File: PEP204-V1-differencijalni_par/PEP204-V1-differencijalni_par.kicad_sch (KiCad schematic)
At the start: 18 parts, among them J1 Screw_Terminal_01x02, J2 Conn_01x02_Pin, J3 Conn_01x02_Pin, J4 Conn_01x02_Pin, J5 Conn_01x02_Pin, Q1 MMBT2222A, Q2 MMBT2222A, Q3 MMBT2222A, U1 CJ432

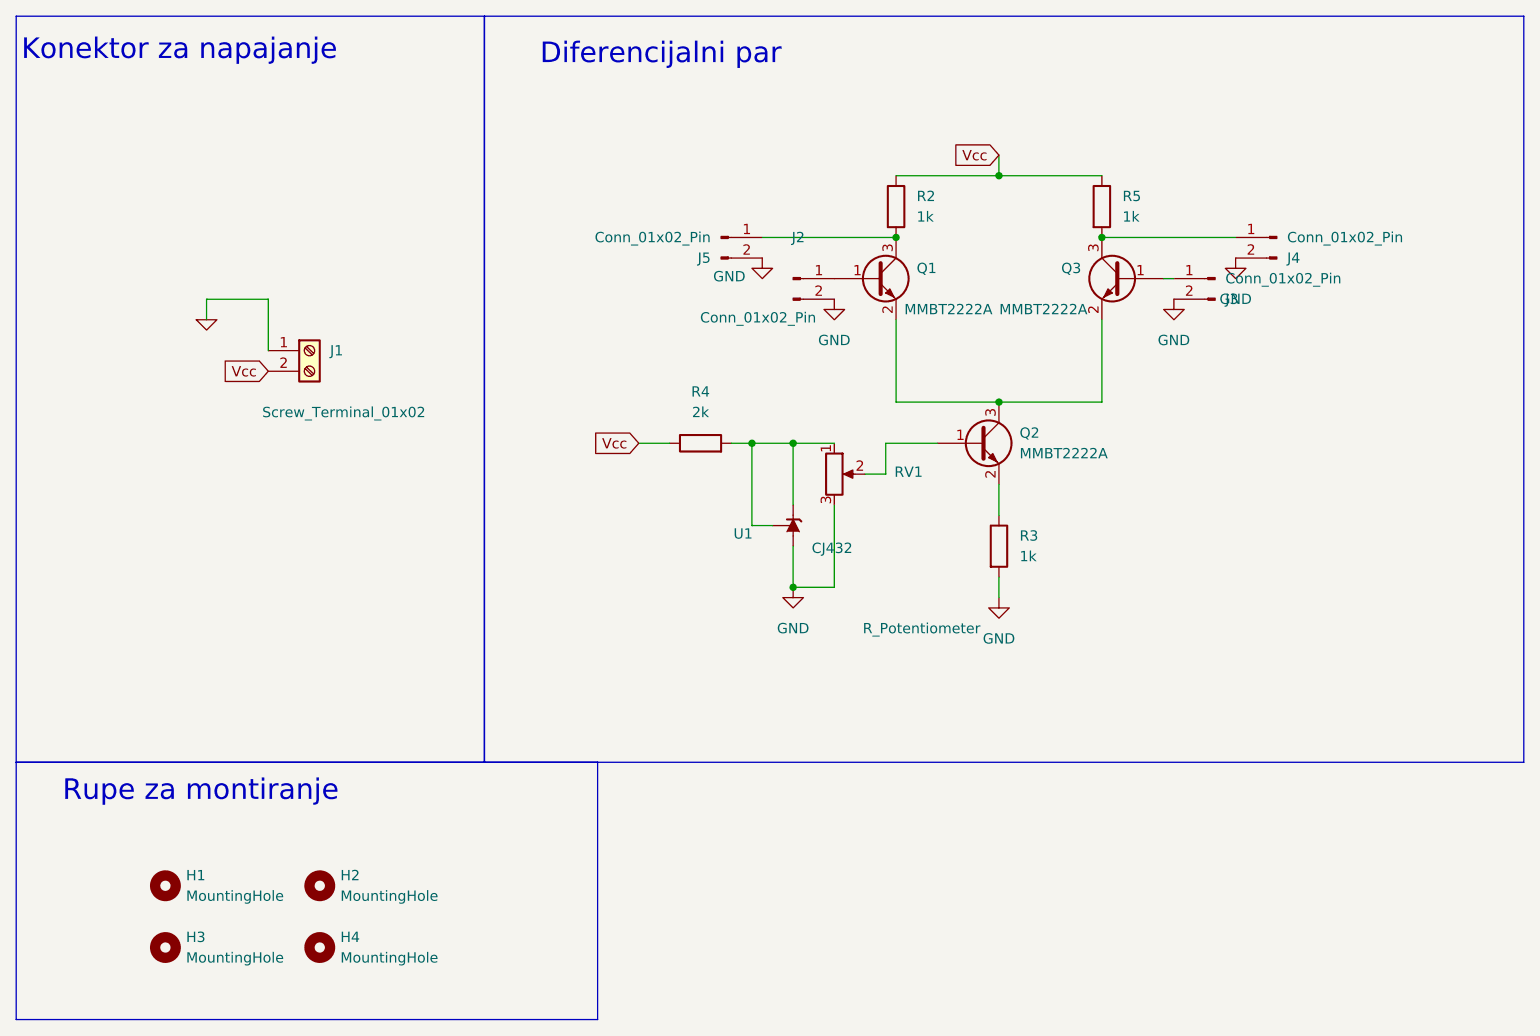
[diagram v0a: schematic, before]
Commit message: PEP201 i PEP204 :)
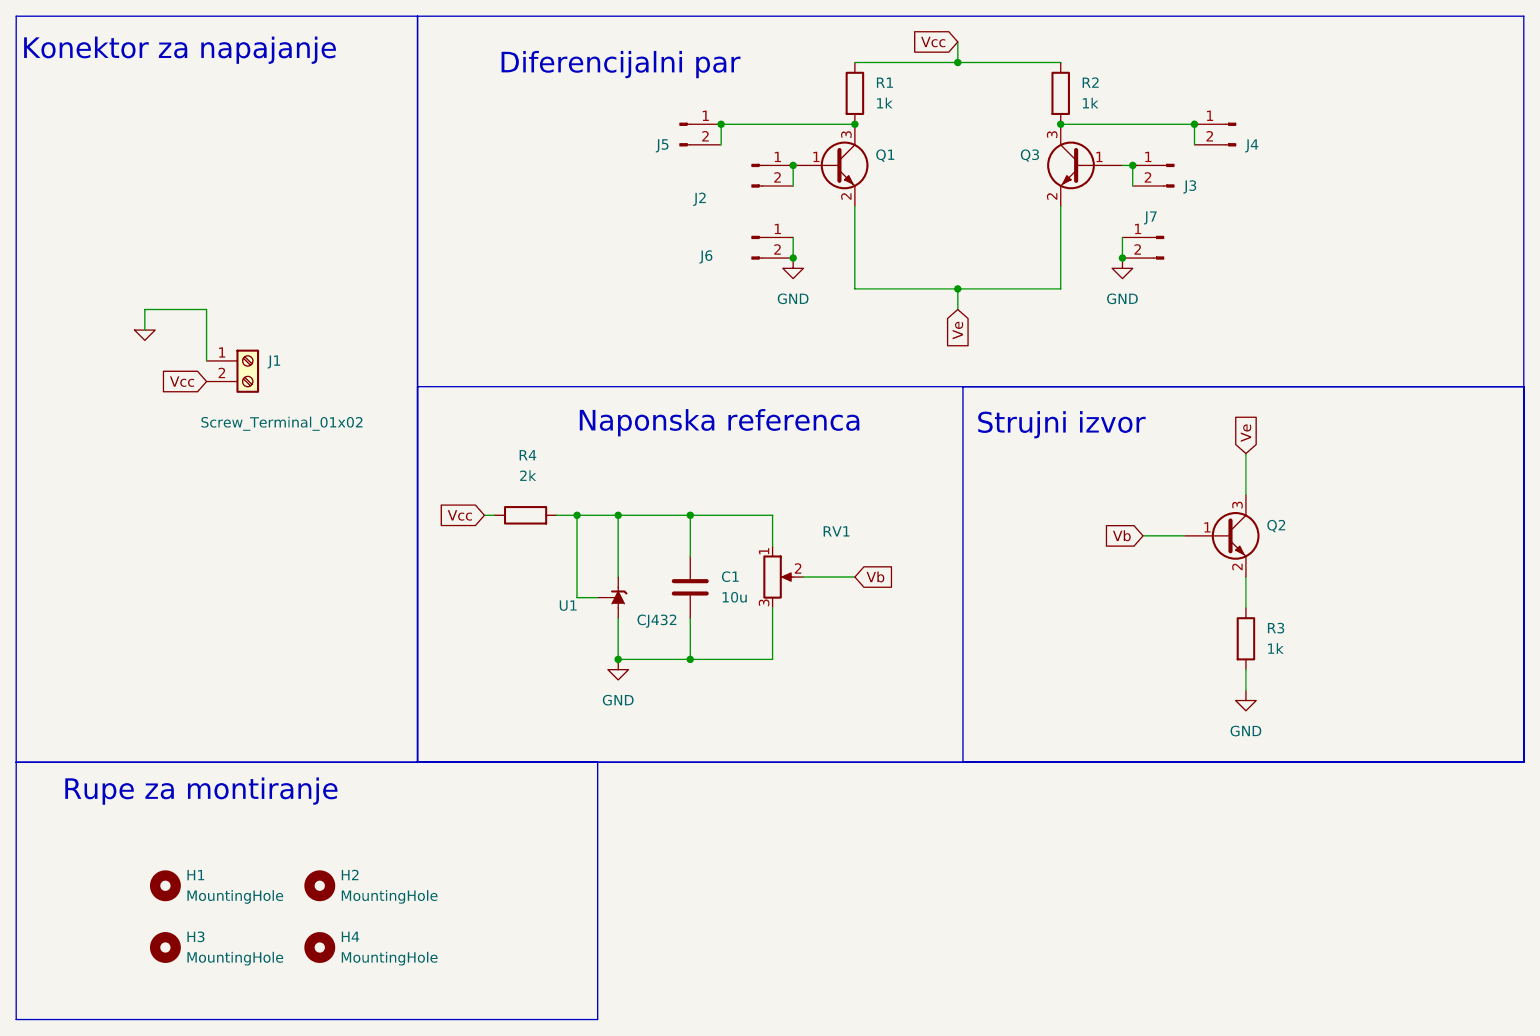
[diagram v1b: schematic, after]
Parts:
- added C1: 10u, PEP_library:C_1206_3216Metric, symbol Device:C
- added J6, J7: Conn_01x02_Pin, PEP_library:PinHeader_1x02_P2.54mm_Vertical, symbol Connector:Conn_01x02_Pin
- Q1, Q2, Q3: LCSC (none) -> C8512
- R1: renamed from R2; LCSC (none) -> C4410
- R2: renamed from R5; LCSC (none) -> C4410
- R3: LCSC (none) -> C4410
- R4: LCSC (none) -> C17944
- U1: LCSC (none) -> C3113
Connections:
- net GND: now also C1.2, J6.1 (Pin_1), J6.2 (Pin_2), J7.1 (Pin_1), J7.2 (Pin_2); no longer J2.2 (Pin_2), J3.2 (Pin_2), J4.2 (Pin_2), J5.2 (Pin_2)
- net at R4.2, RV1.1, U1.1 (REF)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: now also C1.1
- net at J4.1 (Pin_1), Q3.3 (C), R2.2: now also J4.2 (Pin_2)
- net at J2.1 (Pin_1), Q1.1 (B): now also J2.2 (Pin_2)
- net Ve: now reaches Q1.2 (E), Q2.3 (C), Q3.2 (E)
- net at J5.1 (Pin_1), Q1.3 (C), R1.2: now also J5.2 (Pin_2)
- net at J3.1 (Pin_1), Q3.1 (B): now also J3.2 (Pin_2)
- net Vb: now reaches Q2.1 (B), RV1.2
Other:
- note added: "Naponska referenca"
- note added: "Strujni izvor"
- moved on the sheet: J1, J2, J3, J4, J5, Q1, Q2, Q3, R1, R2, R3, R4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
